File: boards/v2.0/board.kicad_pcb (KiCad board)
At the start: 2 copper layers, 95.2 x 86.4 mm, 65 parts, among them J1 KF301-2P, J2 KF301-2P, J3 KF301-2P, J4 KF301-2P, J5 KF301-2P, J6 KF301-2P, P1 Pin Header 2.54mm 01x11, SW1 SW_DPDT_x2, T1 ZMPT101B, T2 ZMPT101B, T3 ZMPT101B, U1 74HC4052N, U2 74HC4052N

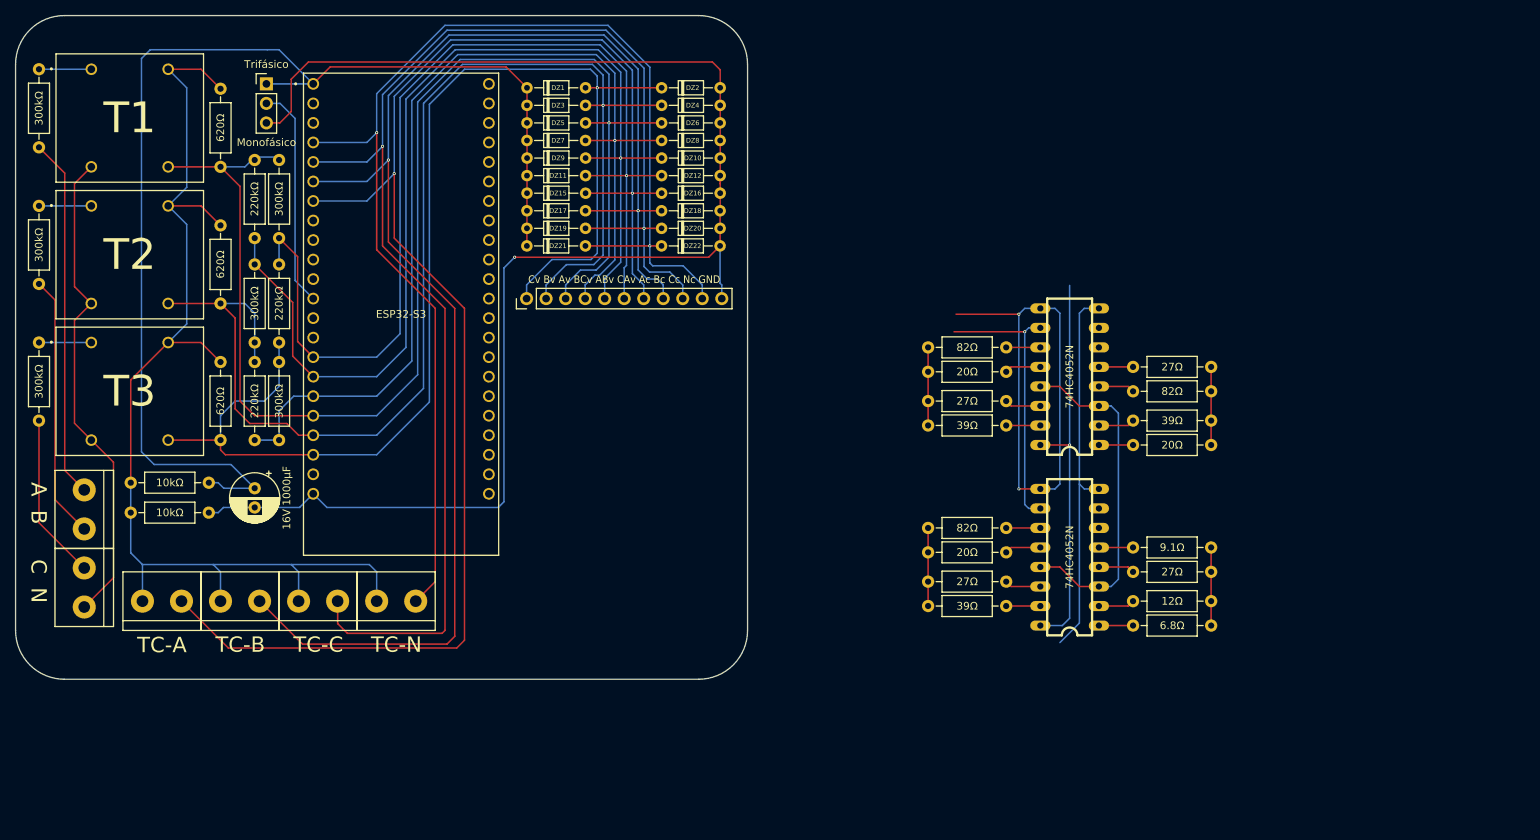
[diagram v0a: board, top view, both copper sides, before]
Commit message: New version of board
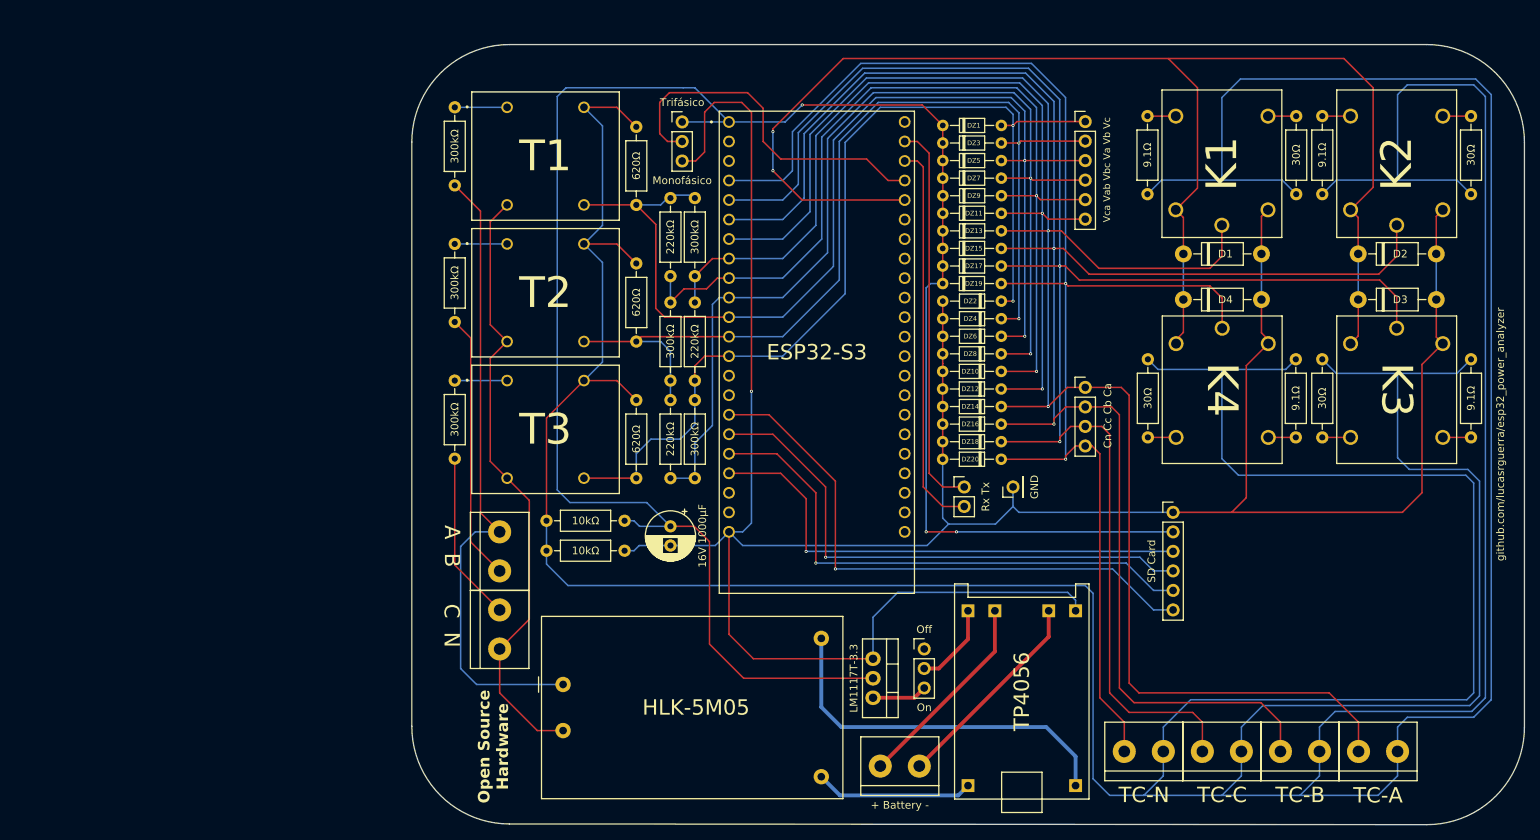
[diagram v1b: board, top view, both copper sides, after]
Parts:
- removed R23, R24, R25: 39Ω, Resistor_THT:R_Axial_DIN0207_L6.3mm_D2.5mm_P10.16mm_Horizontal
- removed R26: 12Ω, Resistor_THT:R_Axial_DIN0207_L6.3mm_D2.5mm_P10.16mm_Horizontal
- removed R27, R28, R29: 82Ω, Resistor_THT:R_Axial_DIN0207_L6.3mm_D2.5mm_P10.16mm_Horizontal
- removed R30: 27Ω, Resistor_THT:R_Axial_DIN0207_L6.3mm_D2.5mm_P10.16mm_Horizontal
- added D1: 1N4007, Diode_THT:D_DO-41_SOD81_P10.16mm_Horizontal, F.Cu at (173.6, 65.3)
- added D2: 1N4007, Diode_THT:D_DO-41_SOD81_P10.16mm_Horizontal, F.Cu at (196.3, 65.3)
- added D3: 1N4007, Diode_THT:D_DO-41_SOD81_P10.16mm_Horizontal, F.Cu at (196.3, 71.2)
- added D4: 1N4007, Diode_THT:D_DO-41_SOD81_P10.16mm_Horizontal, F.Cu at (173.6, 71.2)
- added J1: KF301-2P, TerminalBlock:TerminalBlock_bornier-2_P5.08mm, F.Cu at (134.1, 132.0)
- added K1: SRD-03VDC-SL-C, SnapEDA Library:RELAY_SRD-03VDC-SL-C, F.Cu at (178.6, 53.6)
- added K2: SRD-03VDC-SL-C, SnapEDA Library:RELAY_SRD-03VDC-SL-C, F.Cu at (201.3, 53.6)
- added K3: SRD-03VDC-SL-C, SnapEDA Library:RELAY_SRD-03VDC-SL-C, F.Cu at (201.3, 83.0)
- added K4: SRD-03VDC-SL-C, SnapEDA Library:RELAY_SRD-03VDC-SL-C, F.Cu at (178.6, 83.0)
- added P2: Pin Header, Connector_PinHeader_2.54mm:PinHeader_1x02_P2.54mm_Vertical, F.Cu at (145.0, 95.6)
- added P3: Pin Header, Connector_PinHeader_2.54mm:PinHeader_1x04_P2.54mm_Vertical, F.Cu at (160.8, 82.7)
- added P4: Pin Header, Connector_PinHeader_2.54mm:PinHeader_1x06_P2.54mm_Vertical, F.Cu at (160.8, 48.1)
- added P5: Pin Header, Connector_PinHeader_2.54mm:PinHeader_1x06_P2.54mm_Vertical, F.Cu at (172.2, 98.9)
- added PS1: HLK-5M05, Converter_ACDC:Converter_ACDC_HiLink_HLK-5Mxx, F.Cu at (92.8, 121.3)
- added SW1: SS-12D00G 4mm, Connector_PinHeader_2.54mm:PinHeader_1x03_P2.54mm_Vertical, F.Cu at (139.8, 116.7)
- MCU1: value ESP32-S3-DEVKITC-1U-N8R2 -> ESP32-S3-DEVKITC-1-N16R8; footprint SnapEDA Library:XCVR_ESP32-S3-DEVKITC-1U-N8R2 -> SnapEDA Library:XCVR_ESP32-S3-DEVKITC-1-N8R2
- P1: value Pin Header 2.54mm 01x11 -> Pin Header; footprint Connector_PinHeader_2.54mm:PinHeader_1x11_P2.54mm_Vertical -> Connector_PinHeader_2.54mm:PinHeader_1x01_P2.54mm_Vertical
- R15, R16, R17: value 20Ω -> 9.1Ω
- R18: value 6.8Ω -> 9.1Ω
- R19, R20, R21: value 27Ω -> 30Ω
- R22: value 9.1Ω -> 30Ω
- SW2: renamed from SW1; value SW_DPDT_x2 -> SS-12D00G 4mm
- U1: value 74HC4052N -> TP4056; footprint SnapEDA Library:DIL16 -> SnapEDA Library:TP4056
- U2: value 74HC4052N -> LM1117T-3.3; footprint SnapEDA Library:DIL16 -> Package_TO_SOT_THT:TO-220-3_Vertical
- moved J4 159.4 mm to (196.3, 130.0)
- moved J5 139.3 mm to (186.2, 130.0)
- moved J6 119.2 mm to (176.0, 130.0)
- moved J7 99.2 mm to (165.9, 130.0)
- moved R17 75.0 mm to (211.0, 79.0), turned to -90 degrees
- moved P1 67.9 mm to (151.4, 95.6)
- moved DZ20 65.5 mm to (149.8, 92.0), turned to 180 degrees
- moved DZ18 62.2 mm to (149.8, 89.7), turned to 180 degrees
- moved DZ16 59.1 mm to (149.8, 87.5), turned to 180 degrees
- moved R21 58.9 mm to (191.6, 79.0), turned to -90 degrees
- moved DZ14 56.1 mm to (149.8, 85.2), turned to 180 degrees
- moved J2 55.1 mm to (84.6, 111.6), turned to -90 degrees
- moved R19 54.9 mm to (188.2, 57.5), turned to 90 degrees
- moved J3 54.9 mm to (84.6, 101.5), turned to -90 degrees
- moved DZ15 54.3 mm to (142.2, 64.6)
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- renumbered DZ12 to DZ10, DZ10 to DZ12, DZ15 to DZ13, DZ8 to DZ14, DZ17 to DZ15, DZ6 to DZ16, DZ19 to DZ17, DZ4 to DZ18, DZ21 to DZ19, DZ22 to DZ2, DZ2 to DZ20, DZ20 to DZ4, DZ18 to DZ6, DZ16 to DZ8, J1 to J2, J2 to J3, J3 to J4, J4 to J5, J5 to J6, J6 to J7
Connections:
- DZ10 pad 1: CA Vwave -> AB Vwave
- DZ12 pad 1: AB Vwave -> CA Vwave
- DZ14 pad 1: BC Vwave -> A Cwave
- DZ16 pad 1: A Vwave -> B Cwave
- DZ18 pad 1: B Vwave -> C Cwave
- DZ2 pad 1: N Cwave -> C Vwave
- DZ20 pad 1: C Vwave -> N Cwave
- DZ4 pad 1: C Cwave -> B Vwave
- DZ6 pad 1: B Cwave -> A Vwave
- DZ8 pad 1: A Cwave -> BC Vwave
- J2 pad 1: Line B -> Line C
- J2 pad 2: Line A -> Neutral
- J3 pad 1: Neutral -> Line A
- J3 pad 2: Line C -> Line B
- J4 pad 1: TC A-2 -> A Cwave
- J4 pad 2: A Cwave -> TC A-1
- J5 pad 1: TC A-2 -> B Cwave
- J5 pad 2: B Cwave -> TC A-1
- J6 pad 1: TC A-2 -> C Cwave
- J6 pad 2: C Cwave -> TC A-1
- J7 pad 1: TC A-2 -> N Cwave
- J7 pad 2: N Cwave -> TC A-1
- MCU1 pad J1_10: unconnected-(MCU1-GPIO17-PadJ1_10) -> BC Vwave
- MCU1 pad J1_11: unconnected-(MCU1-GPIO18-PadJ1_11) -> A Vwave
- MCU1 pad J1_12: System Type -> B Vwave
- MCU1 pad J1_13: unconnected-(MCU1-GPIO3-PadJ1_13) -> C Vwave
- MCU1 pad J1_15: CA Vwave -> unconnected-(MCU1-GPIO9-PadJ1_15)
- MCU1 pad J1_16: AB Vwave -> CS
- MCU1 pad J1_17: BC Vwave -> MOSI
- MCU1 pad J1_18: A Vwave -> SCK
- MCU1 pad J1_19: B Vwave -> MISO
- MCU1 pad J1_20: C Vwave -> unconnected-(MCU1-GPIO14-PadJ1_20)
- MCU1 pad J1_8: unconnected-(MCU1-GPIO15-PadJ1_8) -> CA Vwave
- MCU1 pad J1_9: unconnected-(MCU1-GPIO16-PadJ1_9) -> AB Vwave
- MCU1 pad J3_2: unconnected-(MCU1-U0TXD/GPIO43-PadJ3_2) -> UART TX
- MCU1 pad J3_3: unconnected-(MCU1-U0RXD/GPIO44-PadJ3_3) -> UART RX
- MCU1 pad J3_4: Select C-B -> System Type
- MCU1 pad J3_5: Select C-A -> Select C Level
- P1 pad 1: C Vwave -> GND
- R1 pad 2: TC A-2 -> TC A-1
- R15 pad 1: A Cwave -> TC A-1
- R15 pad 2: Net-(U1-X0) -> Net-(K1-PadNC)
- R16 pad 1: B Cwave -> TC A-1
- R16 pad 2: Net-(U1-Y0) -> Net-(K2-PadNC)
- R17 pad 1: C Cwave -> TC A-1
- R17 pad 2: Net-(U2-X0) -> Net-(K3-PadNC)
- R18 pad 1: N Cwave -> TC A-1
- R18 pad 2: Net-(U2-Y0) -> Net-(K4-PadNC)
- R19 pad 1: A Cwave -> TC A-1
- R19 pad 2: Net-(U1-X1) -> Net-(K1-PadNO)
- R2 pad 1: TC A-2 -> TC A-1
- R20 pad 1: B Cwave -> TC A-1
- R20 pad 2: Net-(U1-Y1) -> Net-(K2-PadNO)
- R21 pad 1: C Cwave -> TC A-1
- R21 pad 2: Net-(U2-X1) -> Net-(K3-PadNO)
- R22 pad 1: N Cwave -> TC A-1
- R22 pad 2: Net-(U2-Y1) -> Net-(K4-PadNO)
- R6 pad 2: TC A-2 -> TC A-1
- R7 pad 2: TC A-2 -> TC A-1
- R8 pad 2: TC A-2 -> TC A-1
- T1 pad 4: TC A-2 -> TC A-1
- T2 pad 4: TC A-2 -> TC A-1
- T3 pad 4: TC A-2 -> TC A-1
- U2 pad 1: Net-(U2-Y0) -> GND
- U2 pad 2: Net-(U2-Y2) -> Vcc
- U2 pad 3: TC A-2 -> Net-(SW1A-C)
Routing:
- net TC A-1: track 0.00 -> 810.5 mm
- net TC A-2: track 189.3 -> 0.00 mm
- net Select C Level: track 0.00 -> 183.1 mm, vias 0 -> 2
- net GND: track 244.8 -> 361.9 mm
- net CS: track 0.00 -> 75.0 mm, vias 0 -> 1
- net SCK: track 0.00 -> 70.5 mm, vias 0 -> 1
- net MOSI: track 0.00 -> 70.5 mm, vias 0 -> 1
- net MISO: track 0.00 -> 66.0 mm, vias 0 -> 1
- net Select C-B: track 64.7 -> 0.00 mm, vias 2 -> 0
- net Vcc: track 206.7 -> 264.0 mm, vias 1 -> 3
- net UART RX: track 0.00 -> 50.8 mm
- net UART TX: track 0.00 -> 50.8 mm
- net Net-(PS1--Vout): track 0.00 -> 48.5 mm
- net Line A: track 47.0 -> 83.4 mm
- net B Vwave: track 168.4 -> 132.0 mm, vias 1 -> 2
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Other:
- board size 95.2 x 86.4 mm -> 144.8 x 101.5 mm
- board text added: "Open Source Hardware"
- board text added: "github.com/lucasrguerra/esp32_power_analyzer"
